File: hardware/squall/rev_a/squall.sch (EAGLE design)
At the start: 36 parts, among them J23 TC2030-JLINK-NL, J5 MICRO_USB_B_JST_MC5BR3-M404-4S, J6 HIROSE-DF40C-10DP-0.4V, J7 HIROSE-DF40C-10DP-0.4V, U2 FT232RQ, U3 NRF51822QF, X1 ABS05-32.768KHZ-9-T, X2 16MHz

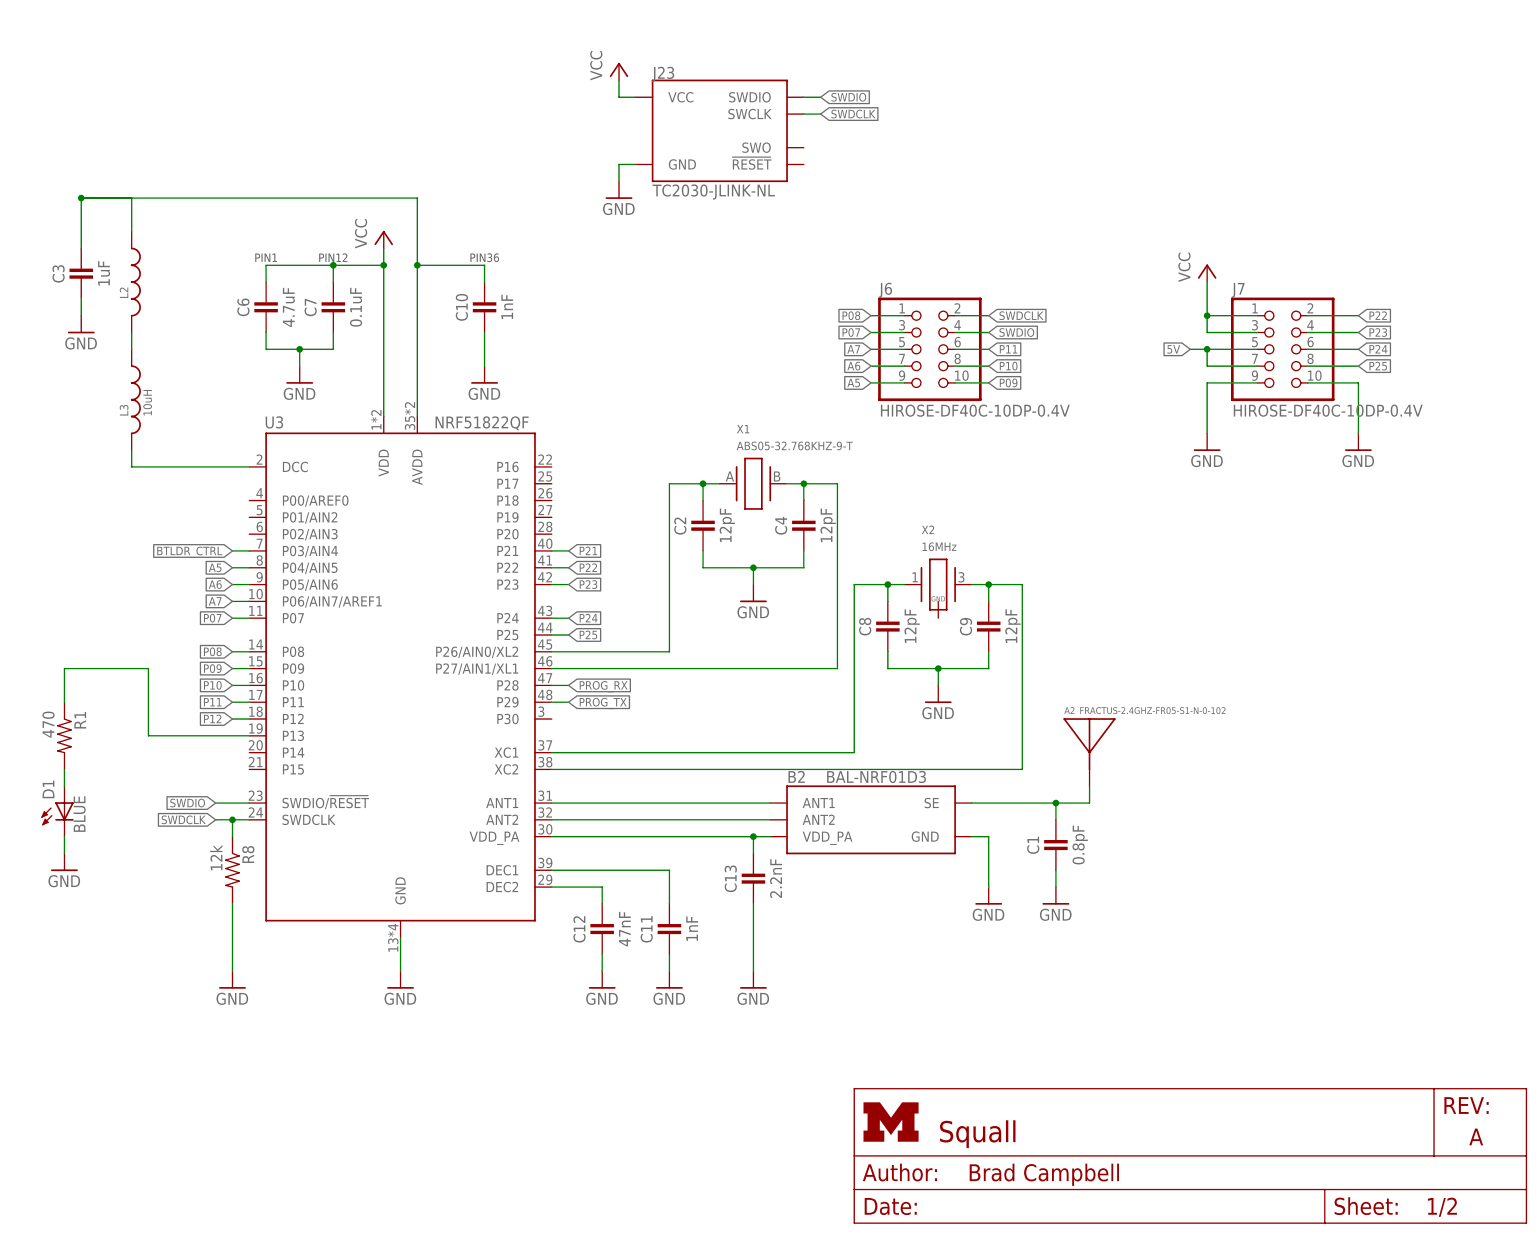
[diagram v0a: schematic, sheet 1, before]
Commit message: getting close, real close to shipping squall
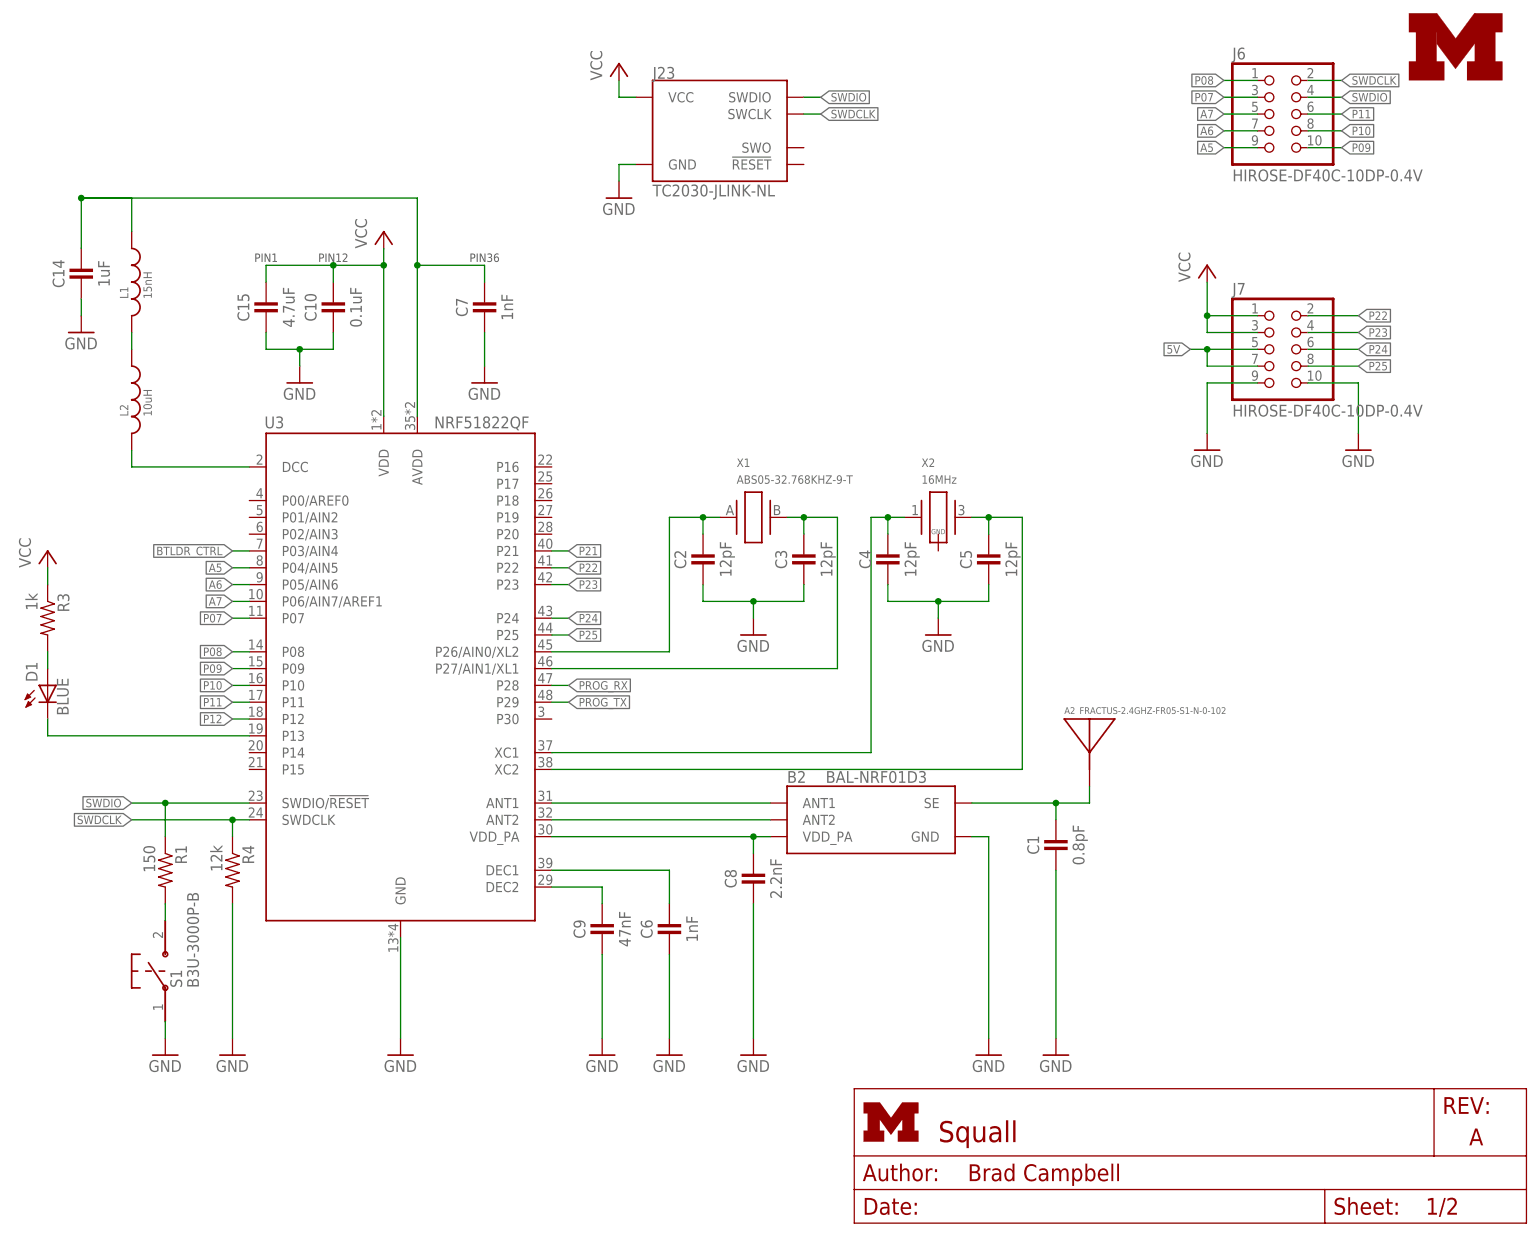
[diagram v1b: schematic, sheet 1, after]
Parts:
- removed C16, C17, C18: 0.1uF, passives:CAPACITOR
- removed L4: (no value), passives:INDUCTOR0402
- added C14: 1uF, passives:CAPACITOR
- added C15: 4.7uF, passives:CAPACITOR
- added C5: 12pF, passives:CAPACITOR
- added L1: 15nH, passives:INDUCTOR0402
- added R3: 1k, passives:RESISTOR
- added S1: B3U-3000P-B, switches:B3U-3000P-B
- C10: value 1nF -> 0.1uF; DIGIKEY 490-1303-1-ND -> 445-4952-1-ND
- C11: value 1nF -> 0.1uF; DIGIKEY 490-1303-1-ND -> 490-1318-6-ND
- C12: value 47nF -> 0.1uF; DIGIKEY 445-1264-1-ND -> 490-1318-6-ND
- C13: value 2.2nF -> 0.1uF; DIGIKEY 490-5419-1-ND -> 490-1318-6-ND
- C3: value 1uF -> 12pF; DIGIKEY 1276-1513-1-ND -> 490-6197-1-ND
- C6: value 4.7uF -> 1nF; DIGIKEY 445-5947-1-ND -> 490-1303-1-ND
- C7: value 0.1uF -> 1nF; DIGIKEY 445-4952-1-ND -> 490-1303-1-ND
- C8: value 12pF -> 2.2nF; DIGIKEY 490-6197-1-ND -> 490-5419-1-ND
- C9: value 12pF -> 47nF; DIGIKEY 490-6197-1-ND -> 445-1264-1-ND
- L2: value (none) -> 10uH; device passives:INDUCTOR0402 -> passives:INDUCTOR0603; DIGIKEY 587-1521-1-ND -> 490-4025-1-ND
- L3: value 10uH -> (none); device passives:INDUCTOR0603 -> passives:INDUCTOR0402; DIGIKEY 490-4025-1-ND -> 445-2979-1-ND
- R1: value 470 -> 150; DIGIKEY RHM470CECT-ND -> RHM150CDCT-ND
- R2: value (none) -> 150; DIGIKEY (none) -> RHM150CDCT-ND
- renumbered R8 to R4
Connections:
- new net N$8: R1.2, S1.P$2
- net 3V3: now also C13.1; no longer C18.1
- net 5V: now also C11.1, L3.1; no longer C16.1, L4.1
- net A1: now also C3.1; no longer C4.1
- net AVDD: now also C14.1, C7.1, L1.1; no longer C10.1, C3.1, L2.1
- net DCC: now also L2.2; no longer L3.2
- net FTDI_VCC: now also C12.1, L3.2; no longer C17.1, L4.2
- net GND: now also C14.2, C15.2, C5.2, S1.P$1; no longer C16.2, C17.2, C18.2, D1.C
- net N$14: now also L1.2, L2.1; no longer L2.2, L3.1
- net N$16: now also C4.1; no longer C8.1
- net N$17: now also C5.1; no longer C9.1
- net N$18: now also C6.1; no longer C11.1
- net N$19: now also C9.1; no longer C12.1
- net N$23: now also R3.2; no longer R1.2
- net N$7: now also D1.C; no longer R1.1
- net SWDIO: now also R1.1
- net VCC: now also C10.1, C15.1, R3.1; no longer C6.1, C7.1
- net VDD_PA: now also C8.1; no longer C13.1
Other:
- moved on the sheet: C10, C2, C3, C4, C6, C7, C8, C9, D1, J6, L2, R1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
